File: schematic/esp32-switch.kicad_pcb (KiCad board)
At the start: 2 copper layers, 100 x 100 mm, 27 parts, among them J1 Direction, J11 Bouton 5v, J17 Bouton Batterie, J2 + - home, J3 a b x y, J4 L R ZL ZR, J5 Joy D, J6 Joy G, J7 Moteur vibration, J8 Batterie, Q1 BC547, U1 ESP32-DevKitC

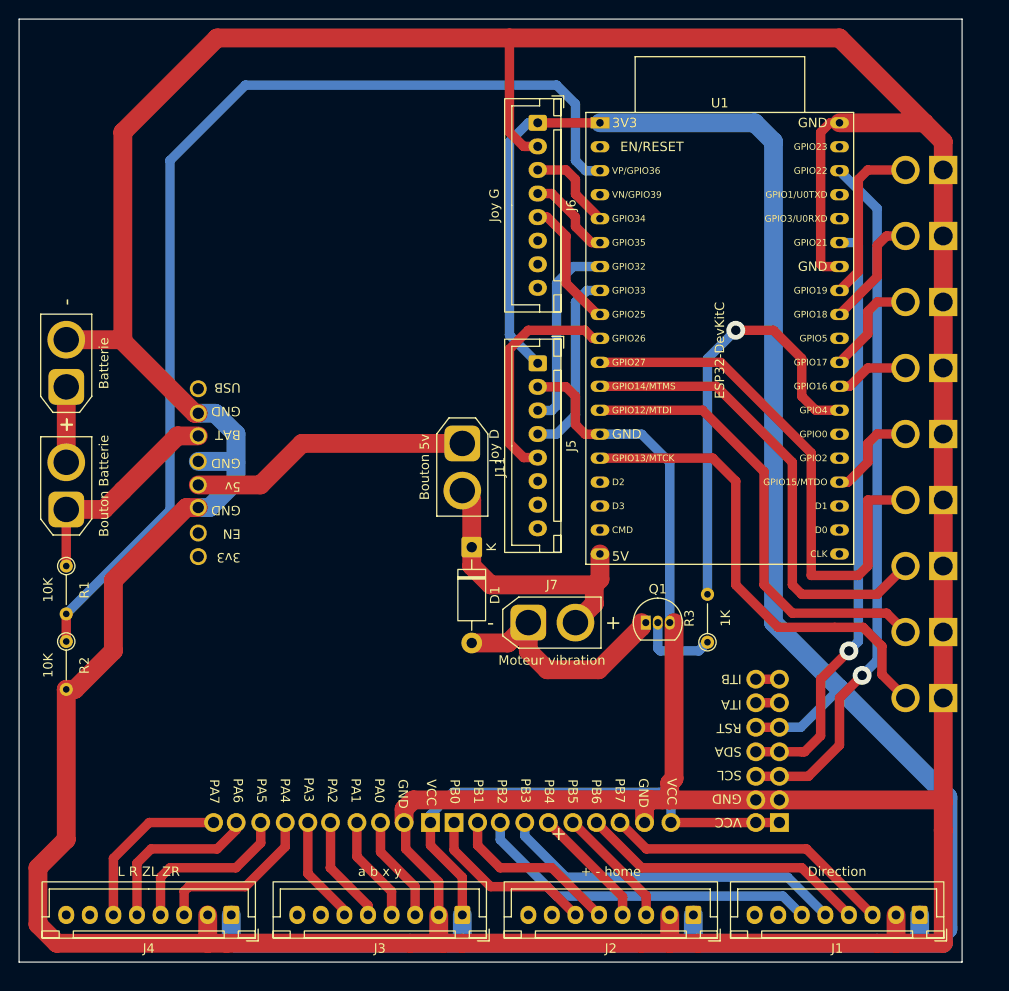
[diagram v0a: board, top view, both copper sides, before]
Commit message: Mise à jour du pcb
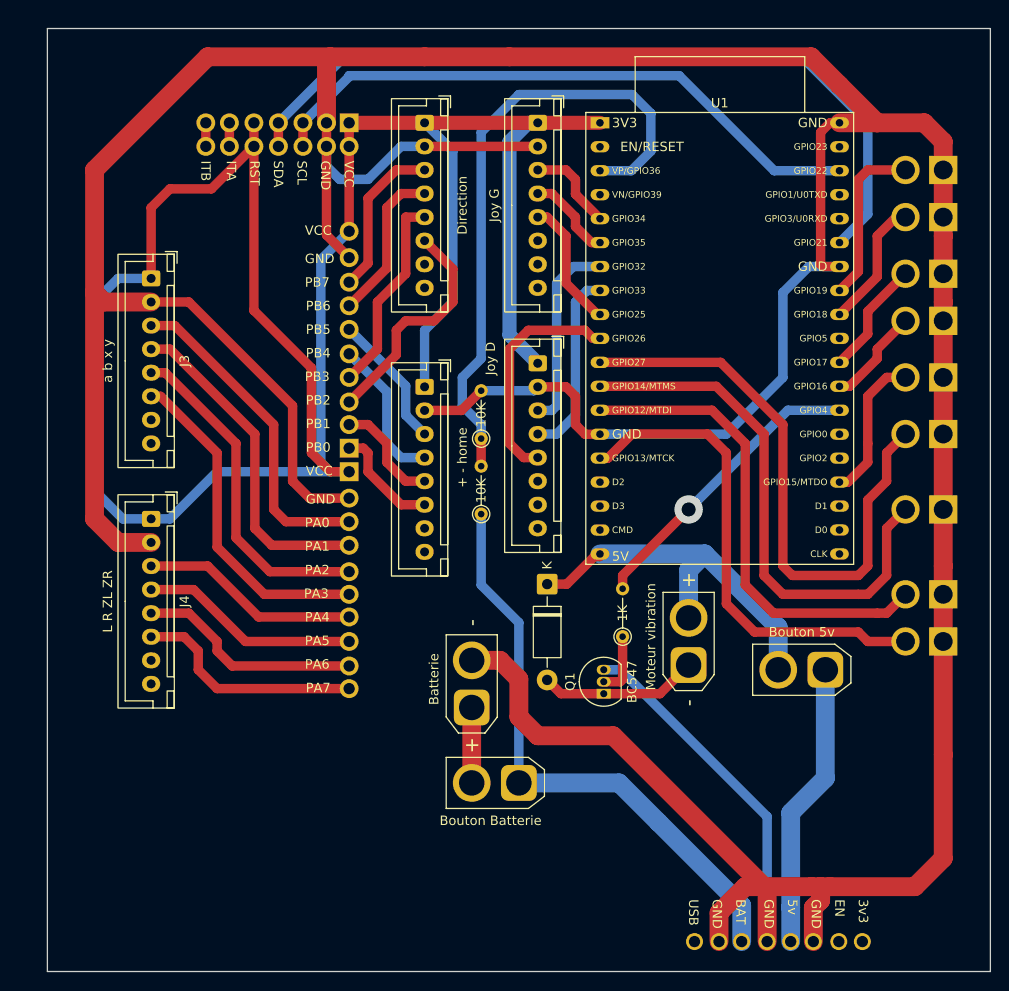
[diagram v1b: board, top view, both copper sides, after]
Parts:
- moved J1 99.1 mm to (182.0, 52.0), turned to -90 degrees
- moved U3 89.1 mm to (156.9, 49.0), turned to 0 degrees
- moved J3 75.1 mm to (153.0, 68.5), turned to -90 degrees
- moved J2 62.8 mm to (182.0, 80.0), turned to -90 degrees
- moved J17 56.1 mm to (192.0, 122.0), turned to 180 degrees
- moved U2 55.4 mm to (237.4, 114.3), turned to -90 degrees
- moved J8 54.8 mm to (187.0, 114.0)
- moved R2 49.0 mm to (188.0, 85.5), turned to 90 degrees
- moved J11 45.4 mm to (224.5, 110.0), turned to 180 degrees
- moved R1 44.3 mm to (188.0, 93.5), turned to 90 degrees
- moved J4 42.9 mm to (153.0, 94.0), turned to -90 degrees
- moved J7 17.6 mm to (210.0, 109.5), turned to 90 degrees
- moved R3 9.02 mm to (203.0, 106.5)
- moved D1 8.91 mm to (195.0, 100.9)
- moved Q1 8.76 mm to (201.0, 112.5), turned to 90 degrees
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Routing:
- net Net-(J1-Pin_2): track 574.2 -> 513.6 mm
- net Net-(J1-Pin_1): track 298.5 -> 245.1 mm
- net Net-(U1-SENSOR_VP/GPIO36/ADC1_CH0): track 111.7 -> 67.8 mm
- net Net-(J17-Pin_1): track 23.2 -> 63.0 mm
- net Net-(J3-Pin_6): track 11.4 -> 35.6 mm
- net Net-(J3-Pin_4): track 11.3 -> 35.5 mm
- net Net-(J3-Pin_5): track 11.5 -> 35.6 mm
- net Net-(J3-Pin_3): track 11.3 -> 34.9 mm
- net Net-(U1-GPIO21): track 63.4 -> 84.7 mm, vias 1 -> 0
- net Net-(J1-Pin_5): track 36.8 -> 21.5 mm
- net Net-(U1-ADC2_CH0/GPIO4): track 46.1 -> 31.7 mm
- net Net-(J1-Pin_4): track 30.8 -> 16.7 mm
- net Net-(J1-Pin_3): track 30.8 -> 17.0 mm
- net Net-(J1-Pin_6): track 37.1 -> 24.7 mm
- net Net-(D1-K): track 30.6 -> 41.2 mm
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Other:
- board text added: "Joy D"
- board text removed: "+"
